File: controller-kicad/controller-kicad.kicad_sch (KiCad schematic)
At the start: 118 parts, among them J1 RJ45_Amphenol_RJMG1BD3B8K1ANR, J10 Conn_01x03_Female, J11 Conn_01x02_Female, J12 Conn_01x01, J13 Conn_01x03_Male, J14 Conn_01x05_Female, J2 Conn_01x02_Female, J3 Conn_01x02_Female, J4 Conn_01x02_Female, J5 Conn_01x02_Female, J6 Conn_01x03_Female, J7 Conn_01x03_Female, J8 Conn_01x03_Female, J9 Conn_01x03_Female, SW1 SW_RST, U1 STM32F407ZETx, U10 IPD60R600, U11 TL431DBZ, U12 AD8495, U13 TLP250, U14 NCP1117-5.0_TO252, U15 NCP1117-3.3_TO252, U2 MCP1416, U3 MCP1416, U4 IPD60R600, U5 IPD60R600, U6 LAN8742, U7 MCP1416, U8 MCP1416, U9 IPD60R600, Y1 25 MHz, Y2 25 MHz

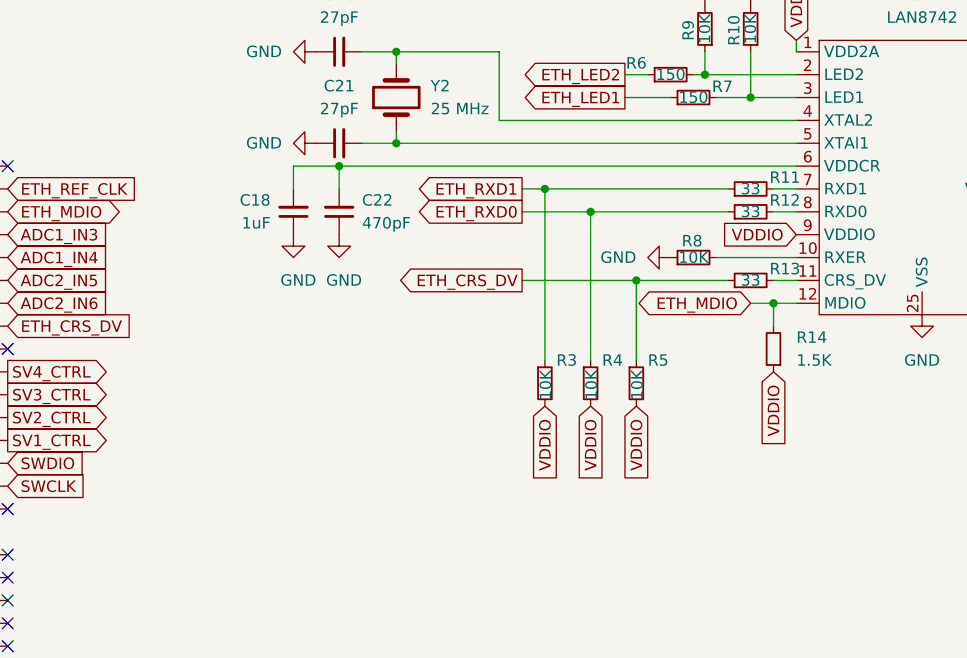
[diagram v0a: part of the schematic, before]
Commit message: More progress on routing
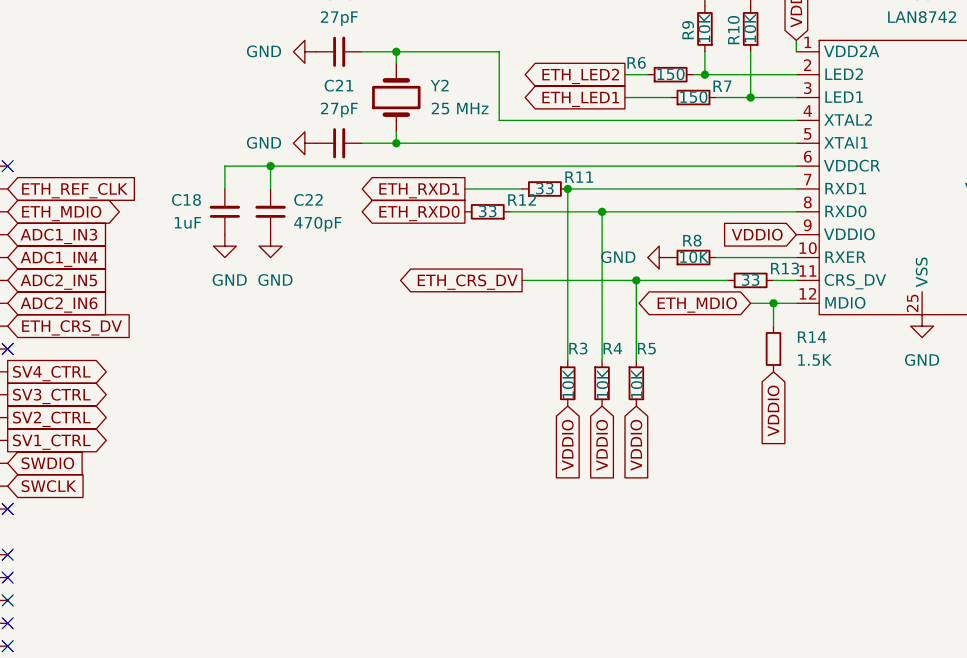
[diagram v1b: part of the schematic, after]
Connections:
- net ETH_RXD0: now also R12.2; no longer R12.1, R4.1
- net ETH_RXD1: no longer R3.1
- net at U6.8 (RXD0): now also R12.1, R4.1; no longer R12.2
- net at R11.2, U6.7 (RXD1): now also R3.1
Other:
- moved on the sheet: C18, C22, R3, R4
